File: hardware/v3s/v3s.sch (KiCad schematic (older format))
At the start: 0 parts

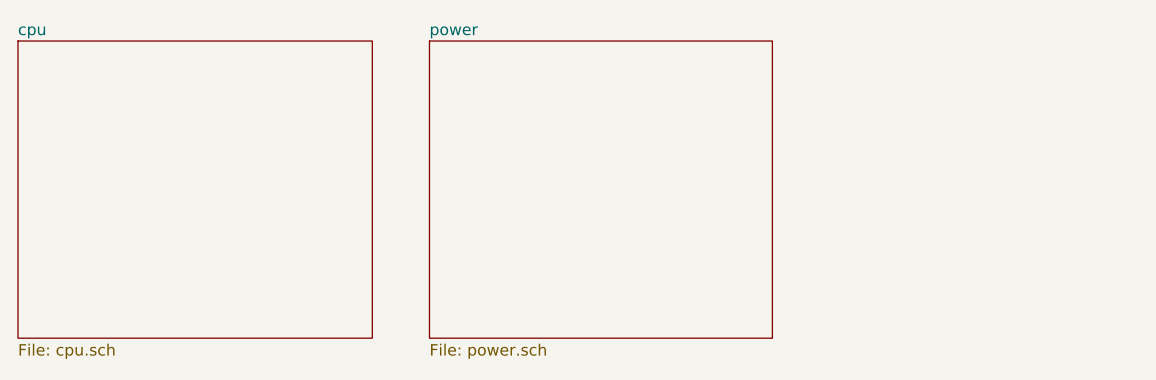
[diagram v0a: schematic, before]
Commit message: working on ...
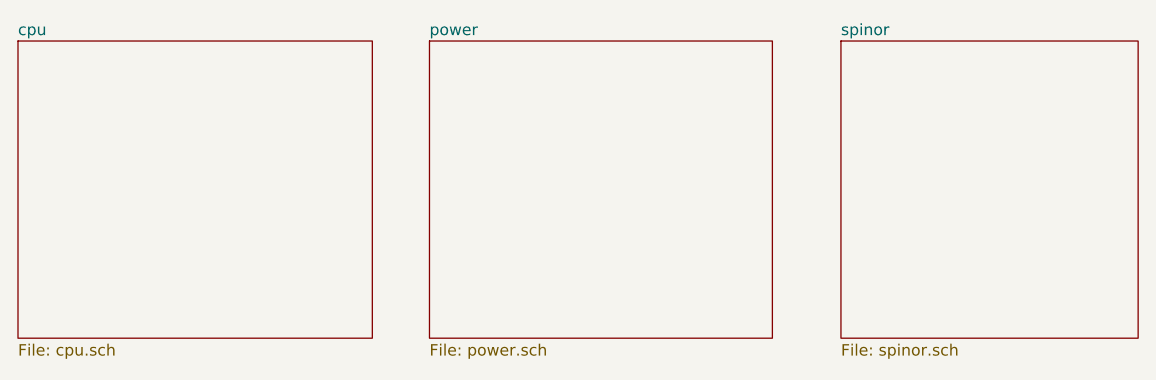
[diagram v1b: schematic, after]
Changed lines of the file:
@@
 $Descr A4 11693 8268
 encoding utf-8
-Sheet 1 3
+Sheet 1 4
 Title ""
 Date ""
@@
 F1 "power.sch" 50
 $EndSheet
+$Sheet
+S 4450 850  1300 1300
+U 5A535D2D
+F0 "spinor" 50
+F1 "spinor.sch" 50
+$EndSheet
 $EndSCHEMATC
